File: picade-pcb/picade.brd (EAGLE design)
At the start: 80 x 50 mm, 60 parts, among them P1JOY 2.54MM-5P-SCREW-TERMINALLOCK, P2JOY 2.54MM-5P-SCREW-TERMINALLOCK

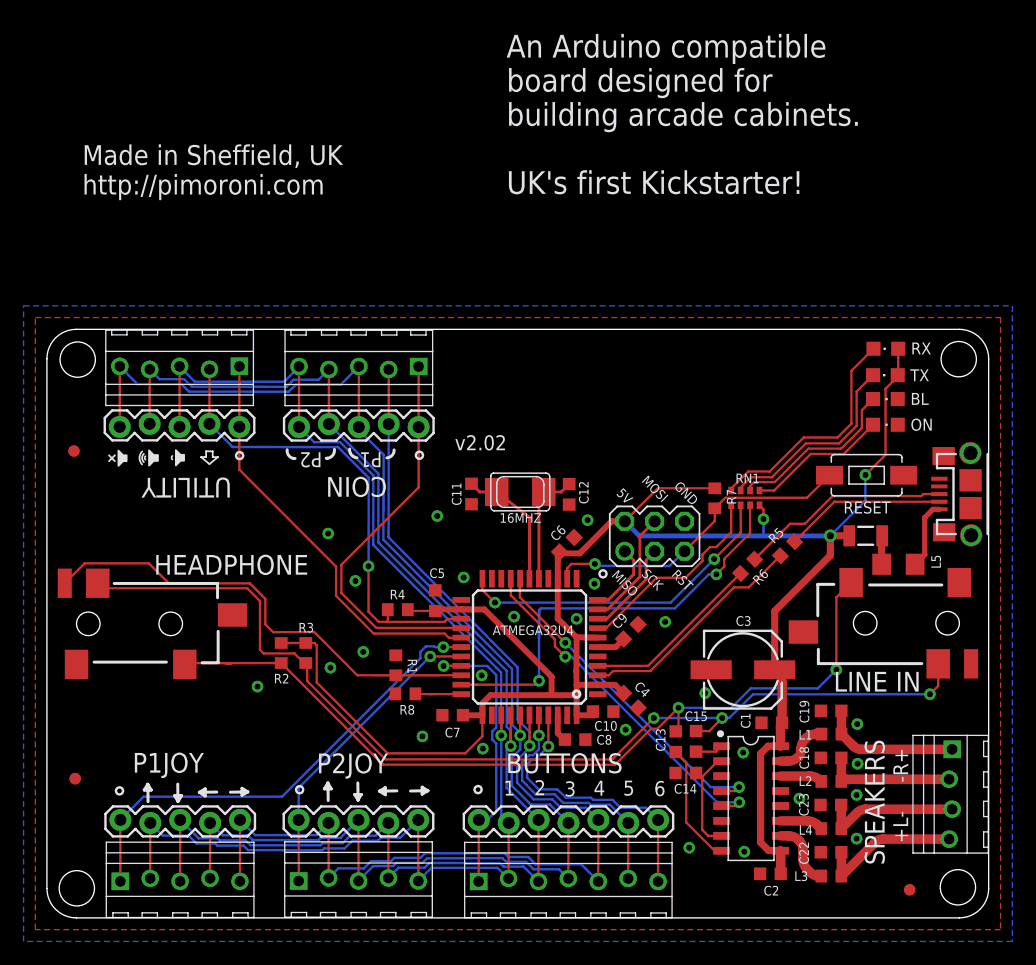
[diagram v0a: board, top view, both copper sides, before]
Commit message: Production candidate
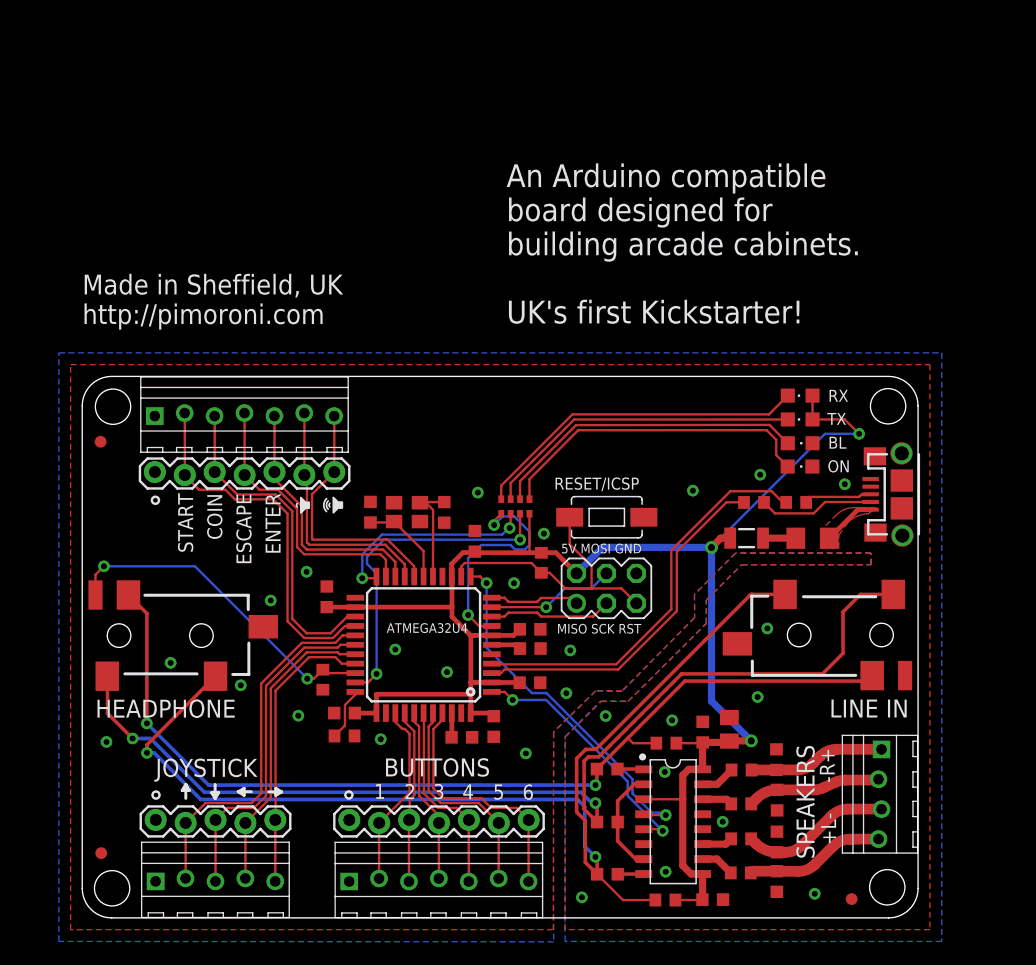
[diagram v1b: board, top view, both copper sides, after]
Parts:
- removed COIN, P1JOY, P2JOY, UTILITY: 2.54MM-5P-SCREW-TERMINALLOCK, pimoroni:2.54MM-5P-SCREW-TERMINAL
- removed JP4, JP5: (no value), SparkFun-Connectors:1X05_LOCK
- removed R4: 47KR, resistor:R0603
- added BUTTONS1: 2.54MM-7P-SCREW-TERMINALLOCK, pimoroni:2.54MM-7P-SCREW-TERMINAL
- added C16: 100nF, resistor:C0805K
- added JOYSTICK: 2.54MM-5P-SCREW-TERMINALLOCK, pimoroni:2.54MM-5P-SCREW-TERMINAL
- 16MHZ: value (none) -> TSX-3225; device adafruit:NX5032 -> pimoroni:TSX-3225
- C3: value 100uF -> 100nF; device resistor:153CLV-0605 -> resistor:C0603K
- JP3: device SparkFun-Connectors:1X05_LOCK -> SparkFun-Connectors:1X07_LOCK
- moved R3 38.8 mm to (49.5, 1.52), turned to 0 degrees
- moved JP3 32.0 mm to (6.16, 37.8)
- moved R2 31.6 mm to (49.6, 14.8), turned to 0 degrees
- moved RESET 22.4 mm to (44.5, 34.0)
- moved RN1 19.6 mm to (36.8, 34.9)
- moved C3 18.4 mm to (38.0, 24.5)
- moved R7 15.7 mm to (39.0, 30.2)
- moved C13 12.7 mm to (44.6, 3.71), turned to 0 degrees
- moved BUTTONS 11.0 mm to (31.6, 3.22)
- moved JP1 11.0 mm to (22.7, 8.19)
- moved C12 10.7 mm to (30.7, 34.4)
- moved F1 10.1 mm to (56.4, 32.3)
- moved 16MHZ 9.77 mm to (27.6, 34.5)
- moved C8 9.62 mm to (32.2, 15.3)
- moved C10 9.38 mm to (34.9, 16.3), turned to 270 degrees
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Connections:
- net IN5 renamed BUTTON5
- net IN6 renamed BUTTON6
- net LINEINL renamed LINEINL+
- net LINEINR renamed LINEINR+
- net N$15 renamed VBUS
- removed net BCOM: ATMEGA32U4.30, BUTTONS.1, JP1.1
- removed net CSCOM: ATMEGA32U4.26, COIN.1, JP4.1
- removed net IN1: ATMEGA32U4.36, BUTTONS.2, COIN.5, JP1.2, JP2.2, JP3.5, JP4.5, JP5.3, P1JOY.2, P2JOY.5, UTILITY.3
- removed net IN2: ATMEGA32U4.37, BUTTONS.3, COIN.4, JP1.3, JP2.3, JP3.4, JP4.4, JP5.4, P1JOY.3, P2JOY.4, UTILITY.4
- removed net IN3: ATMEGA32U4.38, BUTTONS.4, COIN.3, JP1.4, JP2.4, JP3.3, JP4.3, JP5.5, P1JOY.4, P2JOY.3, UTILITY.5
- removed net IN4: ATMEGA32U4.39, BUTTONS.5, COIN.2, JP1.5, JP2.5, JP3.2, JP4.2, P1JOY.5, P2JOY.2
- removed net MODESHIFT: ATMEGA32U4.25, JP5.2, R4.1, UTILITY.2
- removed net P1JCOM: ATMEGA32U4.28, JP2.1, P1JOY.1
- removed net P2JCOM: ATMEGA32U4.29, JP3.1, P2JOY.1
- removed net SHDWN: U$4.3
- removed net UCOM: ATMEGA32U4.27, JP5.1, UTILITY.1
- new net BUTTON1: ATMEGA32U4.36, BUTTONS.2, JP1.2
- new net BUTTON2: ATMEGA32U4.37, BUTTONS.3, JP1.3
- new net BUTTON3: ATMEGA32U4.38, BUTTONS.4, JP1.4
- new net BUTTON4: ATMEGA32U4.39, BUTTONS.5, JP1.5
- new net COIN: ATMEGA32U4.25, BUTTONS1.3, JP3.3
- new net DOWN: ATMEGA32U4.28, JOYSTICK.3, JP2.3
- new net ENTER: ATMEGA32U4.20, BUTTONS1.5, JP3.5
- new net ESCAPE: ATMEGA32U4.21, BUTTONS1.4, JP3.4
- new net LEFT: ATMEGA32U4.29, JOYSTICK.4, JP2.4
- new net LINEIN-: C14.1, HEADPHONES.SLEEVE, LINEIN.SLEEVE
- new net RIGHT: ATMEGA32U4.30, JOYSTICK.5, JP2.5
- new net START: ATMEGA32U4.26, BUTTONS1.2, JP3.2
- new net UP: ATMEGA32U4.27, JOYSTICK.2, JP2.2
- new net VOLUMEDOWN: ATMEGA32U4.19, BUTTONS1.6, JP3.6
- new net VOLUMEUP: ATMEGA32U4.18, BUTTONS1.7, JP3.7
- net 5V: now also C16.1, C3.1, U$4.3; no longer C3.+, R4.2
- net GND: now also 16MHZ.2, 16MHZ.4, BUTTONS.1, BUTTONS1.1, C16.2, C3.2, JOYSTICK.1, JP1.1, JP2.1, JP3.1; no longer C14.1, C3.-, HEADPHONES.SLEEVE, LINEIN.SLEEVE
- net VDOWN: now also ATMEGA32U4.1; no longer ATMEGA32U4.19
- net VUP: now also ATMEGA32U4.12; no longer ATMEGA32U4.18
- net XTAL1: now also 16MHZ.1; no longer 16MHZ.P$2
- net XTAL2: now also 16MHZ.3; no longer 16MHZ.P$1
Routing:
- net IN3: track 125.7 -> 0.00 mm, vias 1 -> 0
- net IN2: track 118.0 -> 0.00 mm, vias 1 -> 0
- net IN1: track 114.1 -> 0.00 mm, vias 1 -> 0
- net IN4: track 99.7 -> 0.00 mm, vias 1 -> 0
- net LINEIN-: track 0.00 -> 89.3 mm, vias 0 -> 2
- net MODESHIFT: track 40.8 -> 0.00 mm, vias 1 -> 0
- net P1JCOM: track 40.6 -> 0.00 mm, vias 1 -> 0
- net UCOM: track 35.0 -> 0.00 mm
- net CSCOM: track 33.4 -> 0.00 mm
- net START: track 0.00 -> 31.3 mm
- net UP: track 0.00 -> 31.2 mm
- net DOWN: track 0.00 -> 28.7 mm
- net COIN: track 0.00 -> 28.3 mm
- net P2JCOM: track 26.3 -> 0.00 mm, vias 1 -> 0
- net LEFT: track 0.00 -> 25.6 mm
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- added copper zone on layer 1, net VBUS
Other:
- board size 80 x 50 mm -> 71 x 46 mm
- board text added: "5V MOSI GND"
- board text added: "MISO SCK RST"
- board text added: "RESET/ICSP"
- board text added: "START COIN ESCAPE ENTER"
- board text added: "v2.03"
- board text removed: "5V"
- board text removed: "GND"
- board text removed: "MISO"
- board text removed: "MOSI"
- board text removed: "P1"
- board text removed: "P2"
- board text removed: "RESET"
- board text removed: "RST"
- board text removed: "SCK"
- board text removed: "v2.00"
- board text removed: "v2.02"
